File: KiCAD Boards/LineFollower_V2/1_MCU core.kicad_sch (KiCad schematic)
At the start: 16 parts, among them IC1 LF33CDT-TRY, IC2 2.4GHz, SW1 TS3625A-HT, SW2 TS3625A-HT

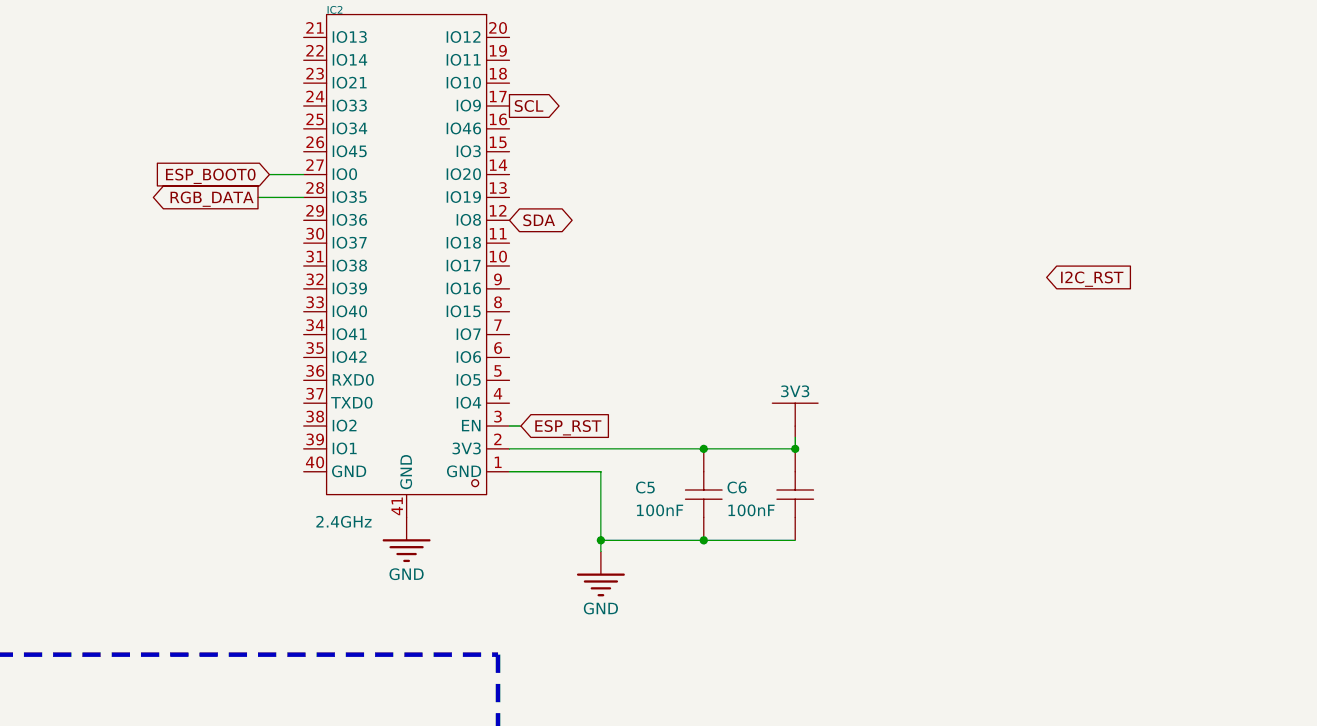
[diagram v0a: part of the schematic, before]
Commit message: more routing
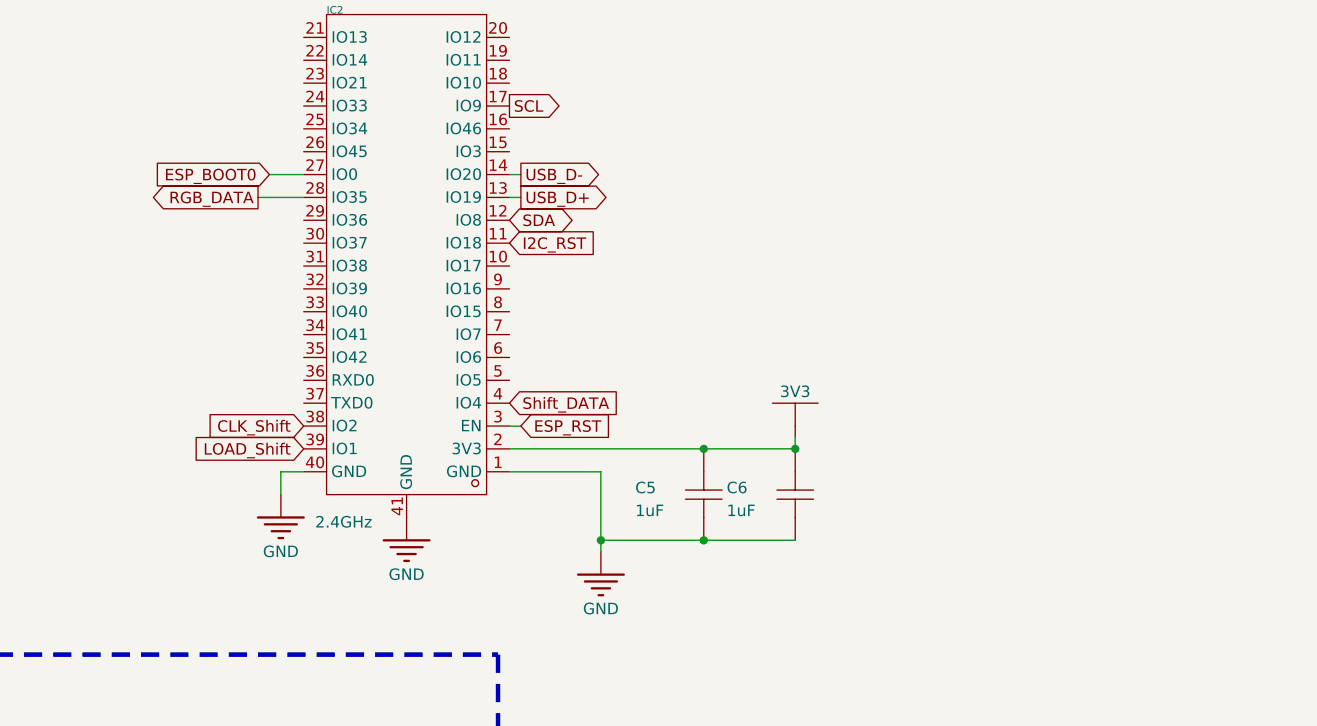
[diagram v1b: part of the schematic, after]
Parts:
- C5, C6: value 100nF -> 1uF
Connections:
- net GND: now also IC2.40 (GND)
- net I2C_RST: now also IC2.11 (IO18)
- net USB_D+: now also IC2.13 (IO19)
- net USB_D-: now also IC2.14 (IO20)
- net CLK_Shift: now reaches IC2.38 (IO2)
- net LOAD_Shift: now reaches IC2.39 (IO1)
- net Shift_DATA: now reaches IC2.4 (IO4)
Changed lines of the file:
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@@
+	(wire
+		(pts
+			(xy 125.73 44.45) (xy 124.46 44.45)
+		)
+		(stroke
+			(width 0)
+			(type default)
+		)
+	)
 	(wire
 		(pts
@@
 	(wire
 		(pts
+			(xy 99.06 77.47) (xy 99.06 74.93)
+		)
+		(stroke
+			(width 0)
+			(type default)
+		)
+	)
+	(wire
+		(pts
 			(xy 49.53 177.8) (xy 49.53 180.34)
 		)
@@
 	(wire
 		(pts
+			(xy 99.06 74.93) (xy 101.6 74.93)
+		)
+		(stroke
+			(width 0)
+			(type default)
+		)
+	)
+	(wire
+		(pts
 			(xy 233.68 151.13) (xy 233.68 153.67)
 		)
@@
 		(pts
 			(xy 80.01 137.16) (xy 85.09 137.16)
+		)
+		(stroke
+			(width 0)
+			(type default)
+		)
+	)
+	(wire
+		(pts
+			(xy 125.73 41.91) (xy 124.46 41.91)
 		)
 		(stroke
@@
 		)
 	)
+	(global_label "LOAD_Shift"
+		(shape input)
+		(at 101.6 72.39 180)
+		(effects
+			(font
+				(size 1.27 1.27)
+			)
+			(justify right)
+		)
+		(property "Intersheetrefs" "${INTERSHEET_REFS}"
+			(at 101.6 72.39 0)
+			(effects
+				(font
+					(size 1.27 1.27)
+				)
+				(hide yes)
+			)
+		)
+	)
 	(global_label "ESP_RST"
 		(shape input)
@@
 		)
 	)
-	(global_label "I2C_RST"
-		(shape input)
-		(at 184.15 53.34 0)
+	(global_label "USB_D-"
+		(shape output)
+		(at 125.73 41.91 0)
 		(effects
 			(font
@@
 		)
 		(property "Intersheetrefs" "${INTERSHEET_REFS}"
-			(at 184.15 53.34 0)
+			(at 125.73 41.91 0)
 			(effects
 				(font
@@
 		)
 	)
+	(global_label "Shift_DATA"
+		(shape input)
+		(at 124.46 67.31 0)
+		(fields_autoplaced yes)
+		(effects
+			(font
+				(size 1.27 1.27)
+			)
+			(justify left)
+		)
+		(property "Intersheetrefs" "${INTERSHEET_REFS}"
+			(at 137.2423 67.31 0)
+			(effects
+				(font
+					(size 1.27 1.27)
+				)
+				(justify left)
+				(hide yes)
+			)
+		)
+	)
 	(global_label "USB_D-"
 		(shape output)
@@
 		)
 	)
+	(global_label "USB_D+"
+		(shape output)
+		(at 125.73 44.45 0)
+		(effects
+			(font
+				(size 1.27 1.27)
+			)
+			(justify left)
+		)
+		(property "Intersheetrefs" "${INTERSHEET_REFS}"
+			(at 125.73 44.45 0)
+			(effects
+				(font
+					(size 1.27 1.27)
+				)
+				(hide yes)
+			)
+		)
+	)
 	(global_label "USB_VBUS"
 		(shape output)
@@
 		)
 	)
+	(global_label "I2C_RST"
+		(shape input)
+		(at 124.46 49.53 0)
+		(effects
+			(font
+				(size 1.27 1.27)
+			)
+			(justify left)
+		)
+		(property "Intersheetrefs" "${INTERSHEET_REFS}"
+			(at 124.46 49.53 0)
+			(effects
+				(font
+					(size 1.27 1.27)
+				)
+				(hide yes)
+			)
+		)
+	)
 	(global_label "USB_VBUS"
 		(shape output)
@@
 		)
 	)
+	(global_label "CLK_Shift"
+		(shape input)
+		(at 101.6 69.85 180)
+		(effects
+			(font
+				(size 1.27 1.27)
+			)
+			(justify right)
+		)
+		(property "Intersheetrefs" "${INTERSHEET_REFS}"
+			(at 101.6 69.85 0)
+			(effects
+				(font
+					(size 1.27 1.27)
+				)
+				(hide yes)
+			)
+		)
+	)
 	(global_label "SCL"
 		(shape output)
@@
 	(symbol
 		(lib_id "Robot druh-easyedapro:Ground-GND")
+		(at 99.06 77.47 0)
+		(unit 1)
+		(exclude_from_sim no)
+		(in_bom yes)
+		(on_board yes)
+		(dnp no)
+		(property "Reference" "#PWR0106"
+			(at 99.06 77.47 0)
+			(effects
+				(font
+					(size 1.27 1.27)
+				)
+				(hide yes)
+			)
+		)
+		(property "Value" "GND"
+			(at 99.06 83.82 0)
+			(effects
+				(font
+					(size 1.27 1.27)
+				)
+			)
+		)
+		(property "Footprint" "Robot druh-easyedapro:"
+			(at 99.06 77.47 0)
+			(effects
+				(font
+					(size 1.27 1.27)
+				)
+				(hide yes)
+			)
+		)
+		(property "Datasheet" ""
+			(at 99.06 77.47 0)
+			(effects
+				(font
+					(size 1.27 1.27)
+				)
+				(hide yes)
+			)
+		)
+		(property "Description" ""
+			(at 99.06 77.47 0)
+			(effects
+				(font
+					(size 1.27 1.27)
+				)
+				(hide yes)
+			)
+		)
+		(pin "1"
+		)
+		(instances
+			(project "LineFollower_V2"
+				(path "/76a20473-53d0-433c-9f05-17cd0a98178a/444a6e75-a2b2-4736-b83b-a01220cf2ff7"
+					(reference "#PWR0106")
+					(unit 1)
+				)
+			)
+		)
+	)
+	(symbol
+		(lib_id "Robot druh-easyedapro:Ground-GND")
 		(at 233.68 153.67 0)
 		(unit 1)
@@
 			)
 		)
-		(property "Value" "100nF"
+		(property "Value" "1uF"
 			(at 148.59 80.01 90)
 			(effects
@@
 			)
 		)
-		(property "Value" "100nF"
+		(property "Value" "1uF"
 			(at 138.43 80.01 90)
 			(effects

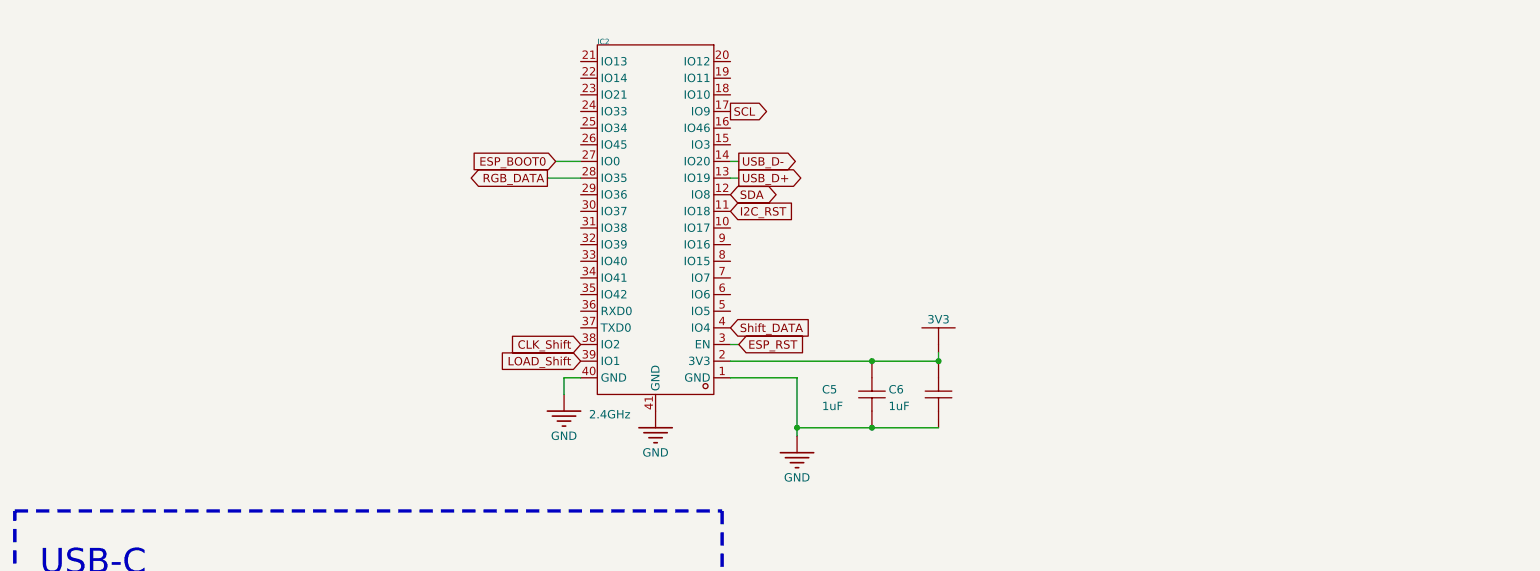
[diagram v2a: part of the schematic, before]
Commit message: v2 board 1.0
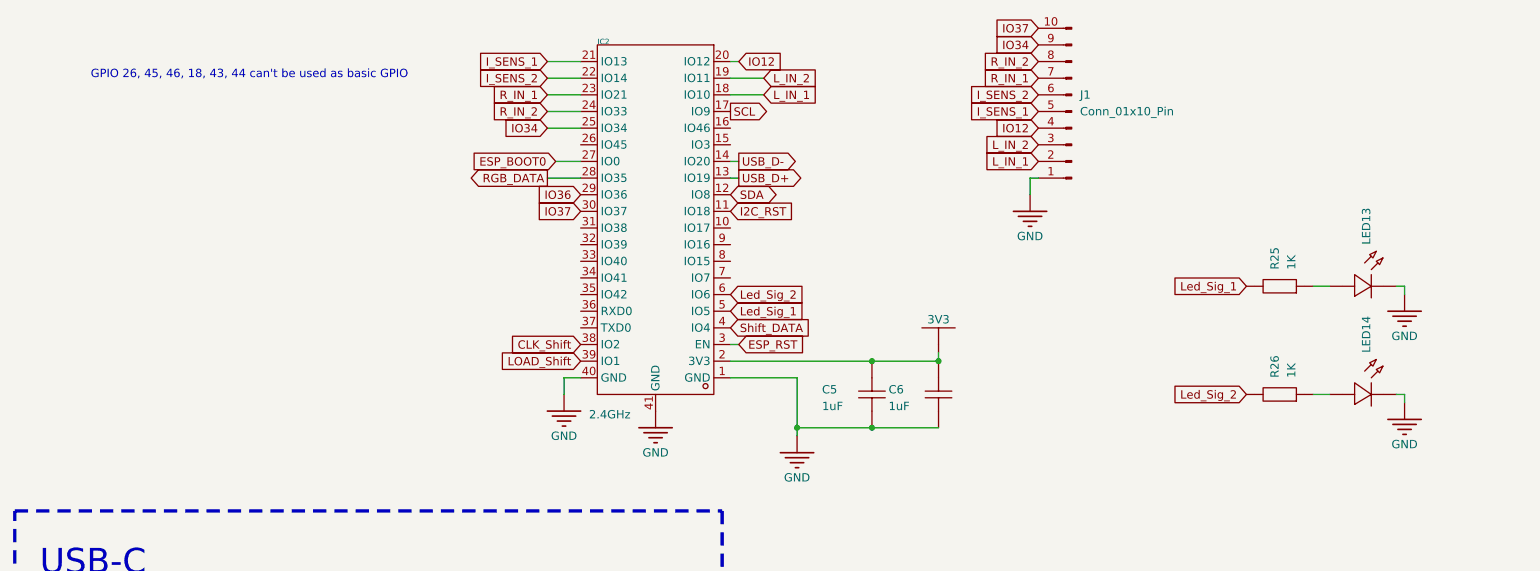
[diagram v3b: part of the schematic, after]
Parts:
- added J1: Conn_01x10_Pin, Connector_PinHeader_2.54mm:PinHeader_1x10_P2.54mm_Vertical, symbol Connector:Conn_01x10_Pin
- added LED13, LED14: ~, easyEDA_footprints:LED0603-RD_GREEN, symbol Robot druh-easyedapro:LED_G
- added R25, R26: 1K, Resistor_SMD:R_0603_1608Metric, symbol Robot druh-easyedapro:Res
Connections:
- net GND: now also J1.1 (Pin_1), LED13.1 (C), LED14.1 (C)
- net L_IN_1: now reaches IC2.18 (IO10)
- net L_IN_1: now also J1.2 (Pin_2)
- net L_IN_2: now reaches IC2.19 (IO11)
- net L_IN_2: now also J1.3 (Pin_3)
- net IO12: now reaches IC2.20 (IO12)
- net IO12: now also J1.4 (Pin_4)
- net I_SENS_1: now reaches IC2.21 (IO13)
- net I_SENS_1: now also J1.5 (Pin_5)
- net I_SENS_2: now reaches IC2.22 (IO14)
- net I_SENS_2: now also J1.6 (Pin_6)
- net R_IN_1: now reaches IC2.23 (IO21)
- net R_IN_1: now also J1.7 (Pin_7)
- net R_IN_2: now reaches IC2.24 (IO33)
- net R_IN_2: now also J1.8 (Pin_8)
- net IO34: now reaches IC2.25 (IO34)
- net IO34: now also J1.9 (Pin_9)
- net IO36: now reaches IC2.29 (IO36)
- net IO37: now reaches IC2.30 (IO37)
- net IO37: now also J1.10 (Pin_10)
- net Led_Sig_1: now reaches IC2.5 (IO5)
- net Led_Sig_1: now also R25.2
- net Led_Sig_2: now reaches IC2.6 (IO6)
- net Led_Sig_2: now also R26.2
- new net: LED13.2 (A), R25.1
- new net: LED14.2 (A), R26.1
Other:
- note added: "GPIO 26, 45, 46, 18, 43, 44 can't be used as basic GPIO"
